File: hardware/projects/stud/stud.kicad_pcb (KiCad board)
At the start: 4 copper layers, 3 parts, among them IC1 R7KA8M2JFLCAC#UC0, IC2 IS42S32160F-7BLI, U2 TAC5242

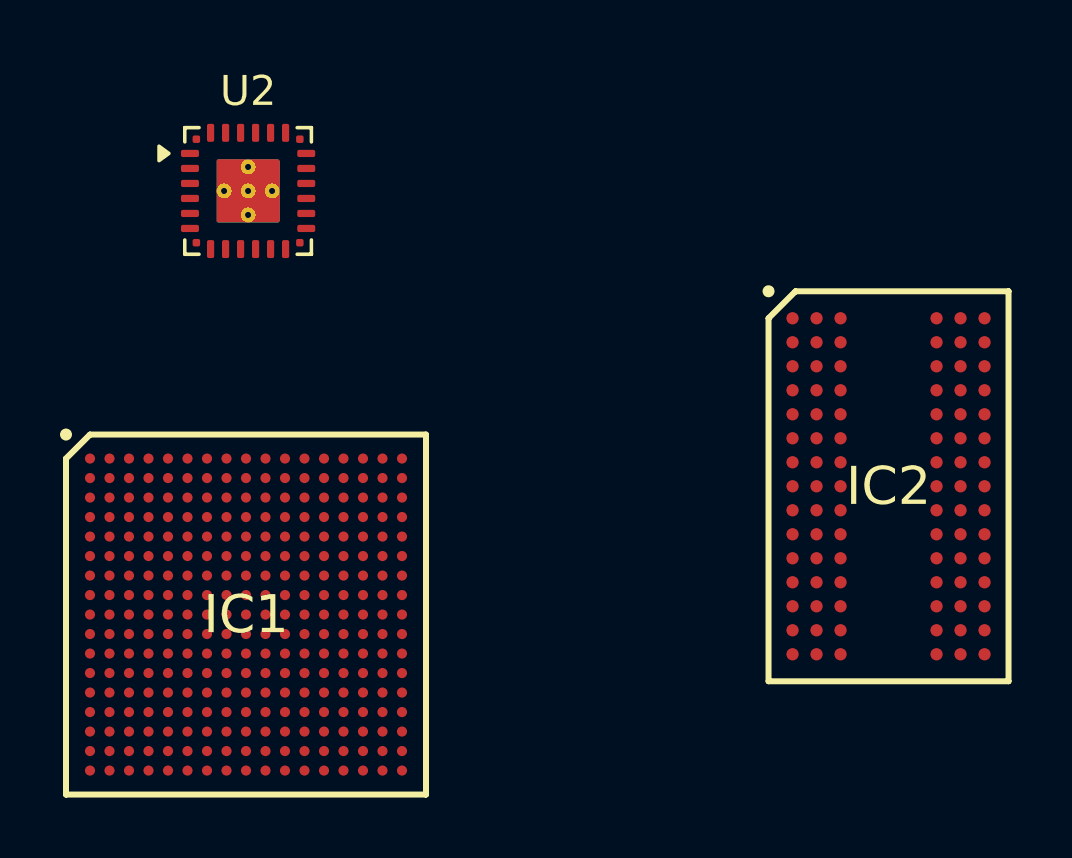
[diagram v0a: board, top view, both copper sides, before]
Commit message: think about routing SDRAM traces
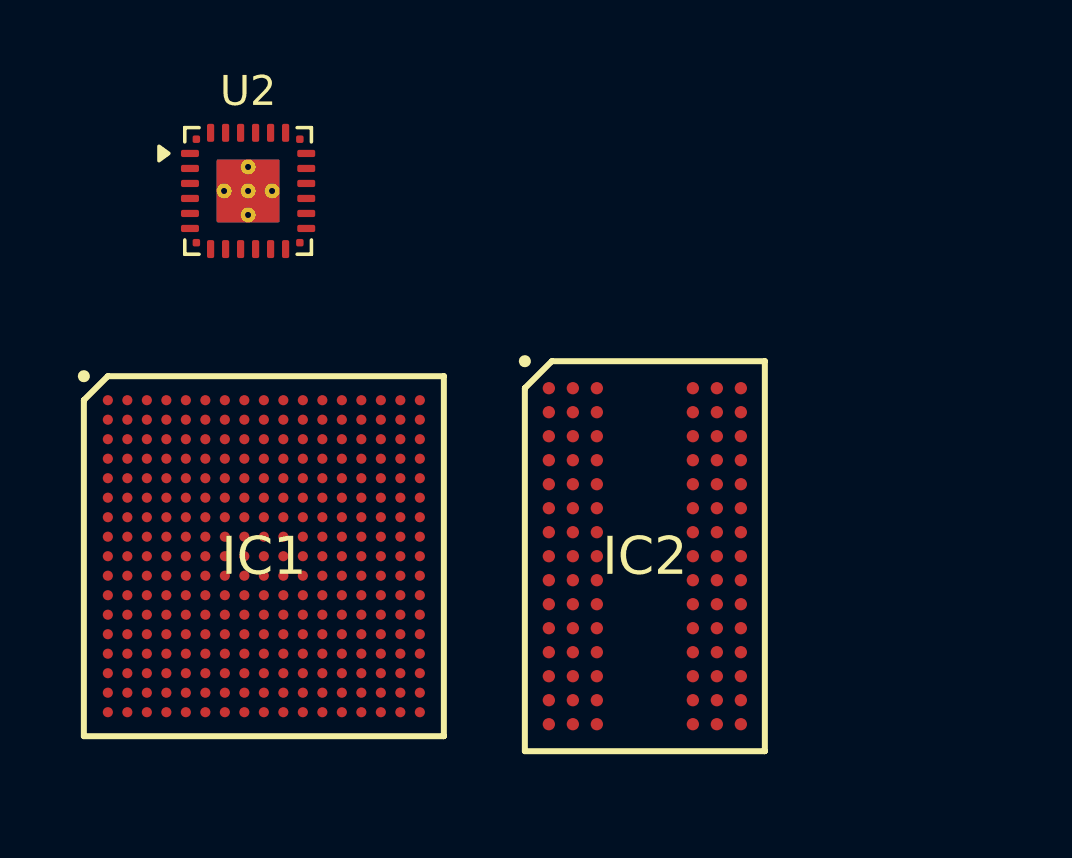
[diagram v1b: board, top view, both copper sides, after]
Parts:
- moved IC2 8.45 mm to (147.3, 109.2)
- moved IC1 2.03 mm to (134.6, 109.2)
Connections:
- IC1 pad L3: unconnected-(IC1-PC04-PadL3) -> DQ26
- IC1 pad L4: unconnected-(IC1-PC09-PadL4) -> DQ21
- IC1 pad L5: unconnected-(IC1-PC05-PadL5) -> DQ25
- IC2 pad A1: unconnected-(IC2-DQ26-PadA1) -> DQ26
- IC2 pad A9: unconnected-(IC2-DQ21-PadA9) -> DQ21
- IC2 pad C3: unconnected-(IC2-DQ25-PadC3) -> DQ25
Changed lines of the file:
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@@
 	(layers
 		(0 "F.Cu" signal)
-		(4 "In1.Cu" signal)
-		(6 "In2.Cu" signal)
+		(4 "In1.Cu" power)
+		(6 "In2.Cu" power)
 		(2 "B.Cu" signal)
 		(9 "F.Adhes" user "F.Adhesive")
@@
 	(footprint "vendor:BGA90C80P9X15_800X1300X120"
 		(layer "F.Cu")
-		(at 155.443 106.889)
+		(at 147.32 109.22)
 		(descr "90L 8x13mm TF-BGA")
 		(tags "Integrated Circuit")
@@
 		(sheetname "/")
 		(sheetfile "stud.kicad_sch")
+		(units
+			(unit
+				(name "A")
+				(pins "A1" "A2" "A3" "A7" "A8" "A9" "B1" "B2" "B3" "B7" "B8" "B9" "C1"
+					"C2" "C3" "C7" "C8" "C9" "D1" "D2" "D3" "D7" "D8" "D9" "E1" "E2" "E3"
+					"E7" "E8" "E9" "F1" "F2" "F3" "F7" "F8" "F9" "G1" "G2" "G3" "G7" "G8"
+					"G9" "H1" "H2" "H3" "H7" "H8" "H9" "J1" "J2" "J3" "J7" "J8" "J9" "K1"
+					"K2" "K3" "K7" "K8" "K9" "L1" "L2" "L3" "L7" "L8" "L9" "M1" "M2" "M3"
+					"M7" "M8" "M9" "N1" "N2" "N3" "N7" "N8" "N9" "P1" "P2" "P3" "P7" "P8"
+					"P9" "R1" "R2" "R3" "R7" "R8" "R9"
+				)
+			)
+		)
 		(solder_mask_margin 0.035)
 		(attr smd)
@@
 			(size 0.41 0.41)
 			(layers "F.Cu" "F.Mask" "F.Paste")
-			(net "unconnected-(IC2-DQ26-PadA1)")
+			(net "DQ26")
 			(pinfunction "DQ26_A1")
 			(pintype "passive")
@@
 			(size 0.41 0.41)
 			(layers "F.Cu" "F.Mask" "F.Paste")
-			(net "unconnected-(IC2-DQ21-PadA9)")
+			(net "DQ21")
 			(pinfunction "DQ21_A9")
 			(pintype "passive")
@@
 			(size 0.41 0.41)
 			(layers "F.Cu" "F.Mask" "F.Paste")
-			(net "unconnected-(IC2-DQ25-PadC3)")
+			(net "DQ25")
 			(pinfunction "DQ25_C3")
 			(pintype "passive")
@@
 	(footprint "vendor:BGA289C65P17X17_1200X1200X138"
 		(layer "F.Cu")
-		(at 134.025 111.165)
+		(at 134.62 109.22)
 		(descr "PLBG0289JA-A")
 		(tags "Integrated Circuit")
@@
 			(size 0.338 0.338)
 			(layers "F.Cu" "F.Mask" "F.Paste")
-			(net "unconnected-(IC1-PC04-PadL3)")
+			(net "DQ26")
 			(pinfunction "PC04_L3")
 			(pintype "passive")
@@
 			(size 0.338 0.338)
 			(layers "F.Cu" "F.Mask" "F.Paste")
-			(net "unconnected-(IC1-PC09-PadL4)")
+			(net "DQ21")
 			(pinfunction "PC09_L4")
 			(pintype "passive")
@@
 			(size 0.338 0.338)
 			(layers "F.Cu" "F.Mask" "F.Paste")
-			(net "unconnected-(IC1-PC05-PadL5)")
+			(net "DQ25")
 			(pinfunction "PC05_L5")
 			(pintype "passive")
